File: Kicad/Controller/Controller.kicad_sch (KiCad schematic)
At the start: 3 parts

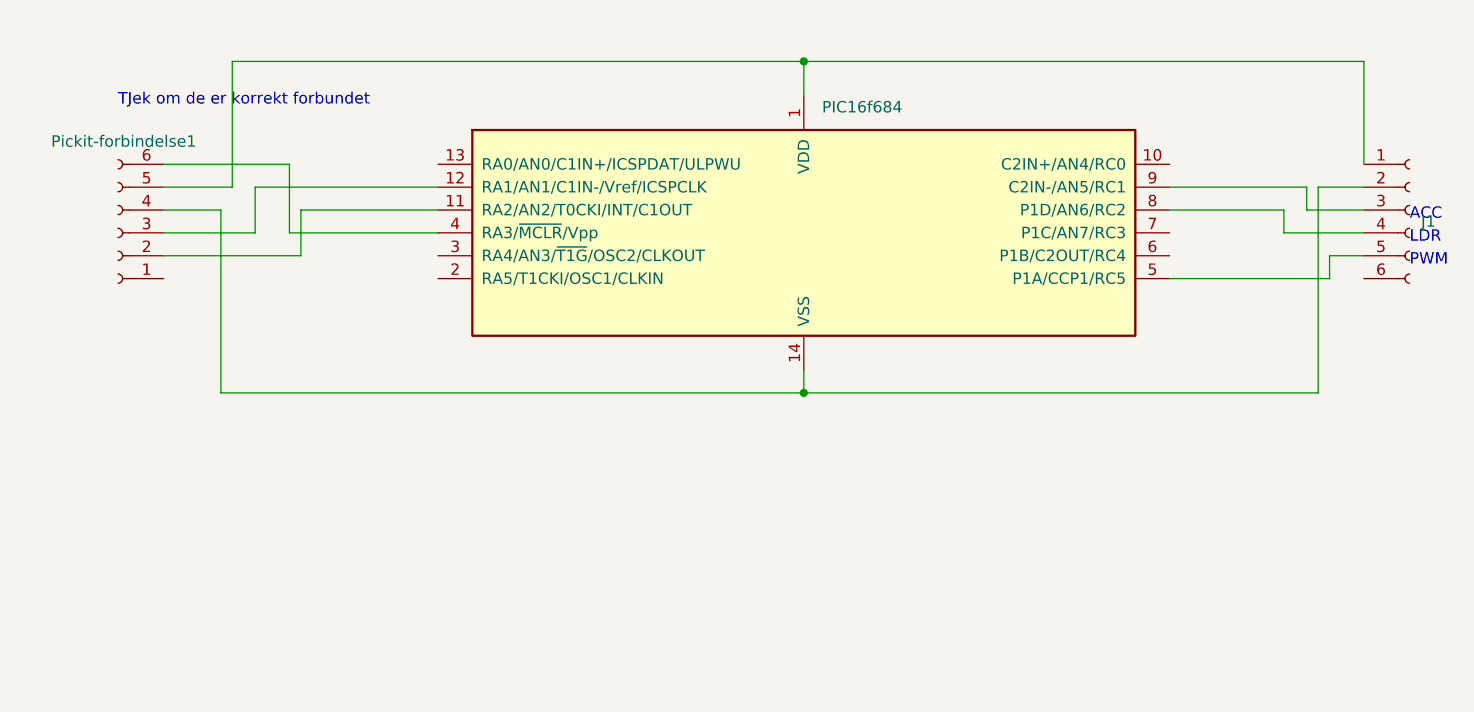
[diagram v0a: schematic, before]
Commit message: Update
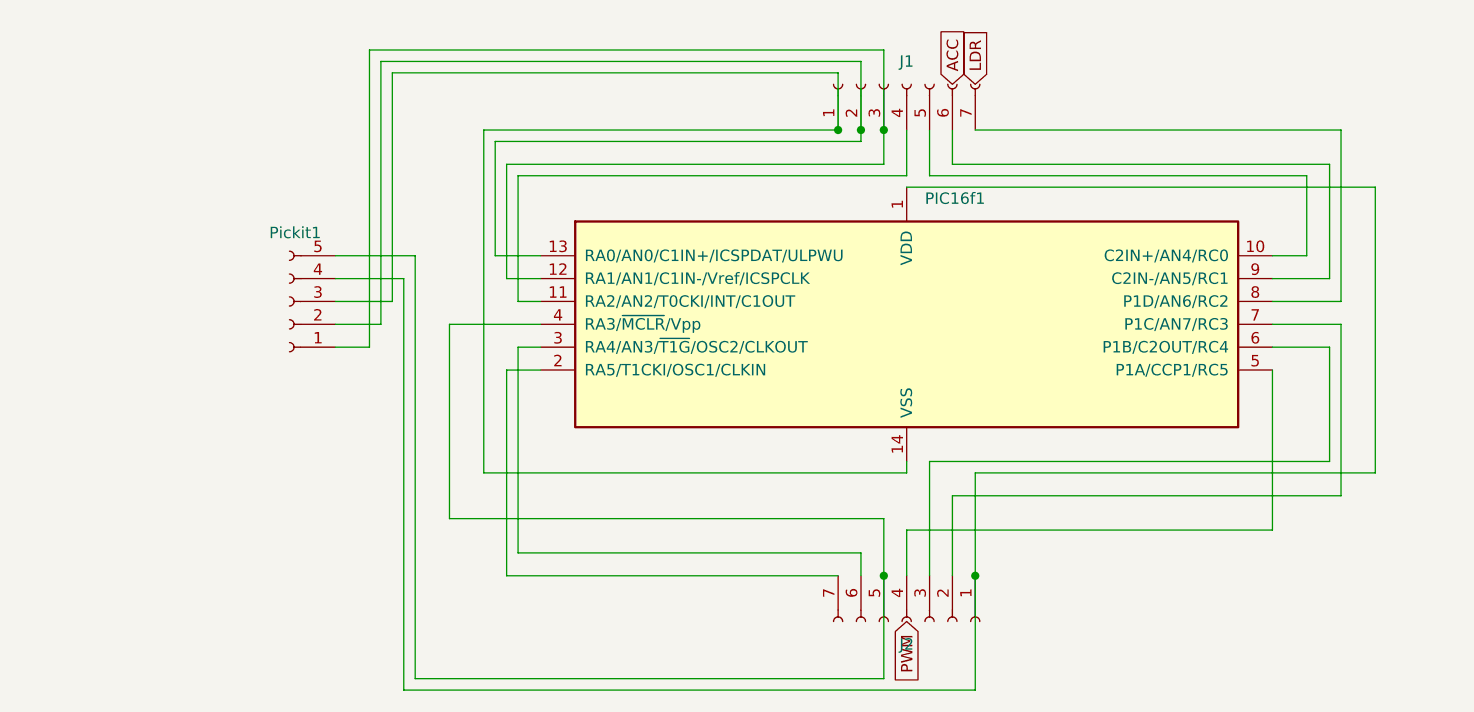
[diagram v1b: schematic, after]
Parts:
- removed J1: (no value), symbol Connector:Conn_01x06_Female
- removed PIC16f684: PIC16F684-IP, Package_DIP:DIP-14_W7.62mm_Socket, symbol MCU_Microchip_PIC16:PIC16F684-IP
- removed Pickit-forbindelse1: Pickit forbindelse, Connector_PinHeader_1.00mm:PinHeader_1x06_P1.00mm_Vertical, symbol Connector:Conn_01x06_Female
- added J1, J2: Conn_01x07_Female, Connector_PinHeader_1.00mm:PinHeader_1x07_P1.00mm_Vertical, symbol Connector:Conn_01x07_Female
- added PIC16f1: PIC16F684-IP, Package_DIP:DIP-14_W7.62mm_Socket, symbol MCU_Microchip_PIC16:PIC16F684-IP
- added Pickit1: Conn_01x05_Female, Connector_PinHeader_1.00mm:PinHeader_1x05_P1.00mm_Vertical, symbol Connector:Conn_01x05_Female
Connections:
- new net: J1.1 (Pin_1), PIC16f1.14 (VSS), Pickit1.3 (Pin_3)
- new net: J1.2 (Pin_2), PIC16f1.13 (RA0/AN0/C1IN+/ICSPDAT/ULPWU), Pickit1.2 (Pin_2)
- new net: J1.3 (Pin_3), PIC16f1.12 (RA1/AN1/C1IN-/Vref/ICSPCLK), Pickit1.1 (Pin_1)
- new net: J1.4 (Pin_4), PIC16f1.11 (RA2/AN2/T0CKI/INT/C1OUT)
- new net: J1.5 (Pin_5), PIC16f1.10 (C2IN+/AN4/RC0)
- new net: J1.6 (Pin_6), PIC16f1.9 (C2IN-/AN5/RC1)
- new net: J1.7 (Pin_7), PIC16f1.8 (P1D/AN6/RC2)
- new net: J2.1 (Pin_1), PIC16f1.1 (VDD), Pickit1.4 (Pin_4)
- new net: J2.7 (Pin_7), PIC16f1.2 (RA5/T1CKI/OSC1/CLKIN)
- new net: J2.6 (Pin_6), PIC16f1.3 (RA4/AN3/~{T1G}/OSC2/CLKOUT)
- new net: J2.5 (Pin_5), PIC16f1.4 (RA3/~{MCLR}/Vpp), Pickit1.5 (Pin_5)
- new net: J2.4 (Pin_4), PIC16f1.5 (P1A/CCP1/RC5)
- new net: J2.3 (Pin_3), PIC16f1.6 (P1B/C2OUT/RC4)
- new net: J2.2 (Pin_2), PIC16f1.7 (P1C/AN7/RC3)
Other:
- note removed: "ACC"
- note removed: "LDR"
- note removed: "PWM"
- note removed: "TJek om de er korrekt forbundet"
